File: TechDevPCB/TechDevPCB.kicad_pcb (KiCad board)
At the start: 2 copper layers, 80.8 x 104.3 mm, 51 parts, among them J1 Screw_Terminal_01x02, J10 Conn_01x05_Pin, J11 Conn_01x01_Socket, J12 Screw_Terminal_01x04, J13 Conn_01x01_Socket, J14 Conn_01x01_Socket, J15 Conn_01x01_Socket, J16 Conn_01x01_Socket, J17 Conn_01x01_Socket, J18 Conn_01x01_Socket, J19 Conn_01x01_Socket, J2 Screw_Terminal_01x02, J20 Conn_01x01_Socket, J21 Conn_01x01_Socket, J22 Conn_01x01_Socket, J23 Conn_01x01_Socket, J24 Conn_01x01_Socket, J25 Conn_01x01_Socket, J26 Conn_01x01_Socket, J27 Conn_01x01_Socket, J28 Conn_01x01_Socket, J29 Conn_01x01_Socket, J3 Conn_01x02_Pin, J30 Conn_01x01_Socket, J31 Conn_01x01_Socket, J4 Screw_Terminal_01x04, J5 Conn_01x02_Pin, J6 Conn_01x05_Pin, J7 Conn_01x04_Pin, J8 Conn_01x05_Pin, J9 Conn_01x05_Pin, U1 DRV8825_STEPPER_MOTOR_DRIVER_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, U2 DRV8825_STEPPER_MOTOR_DRIVER_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, U3 XL6009 Boost Converter

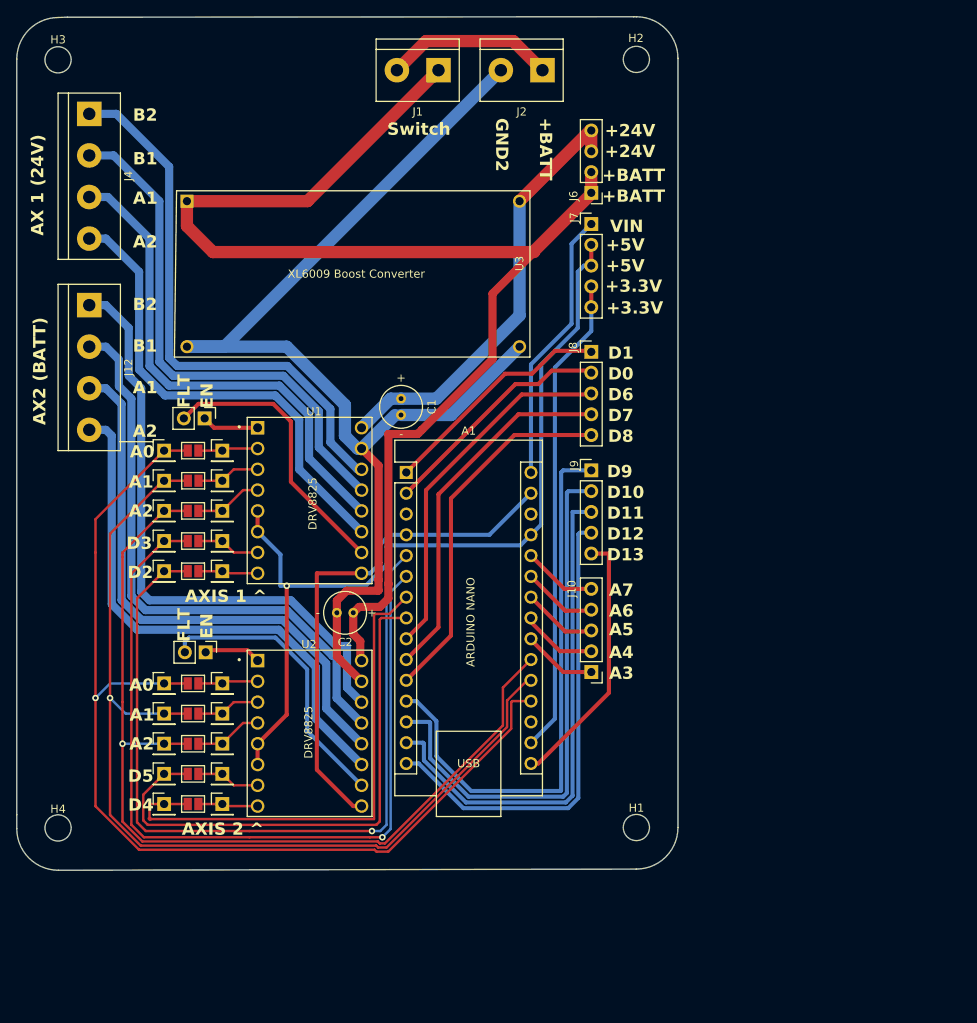
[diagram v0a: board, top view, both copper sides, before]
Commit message: PCB Updates
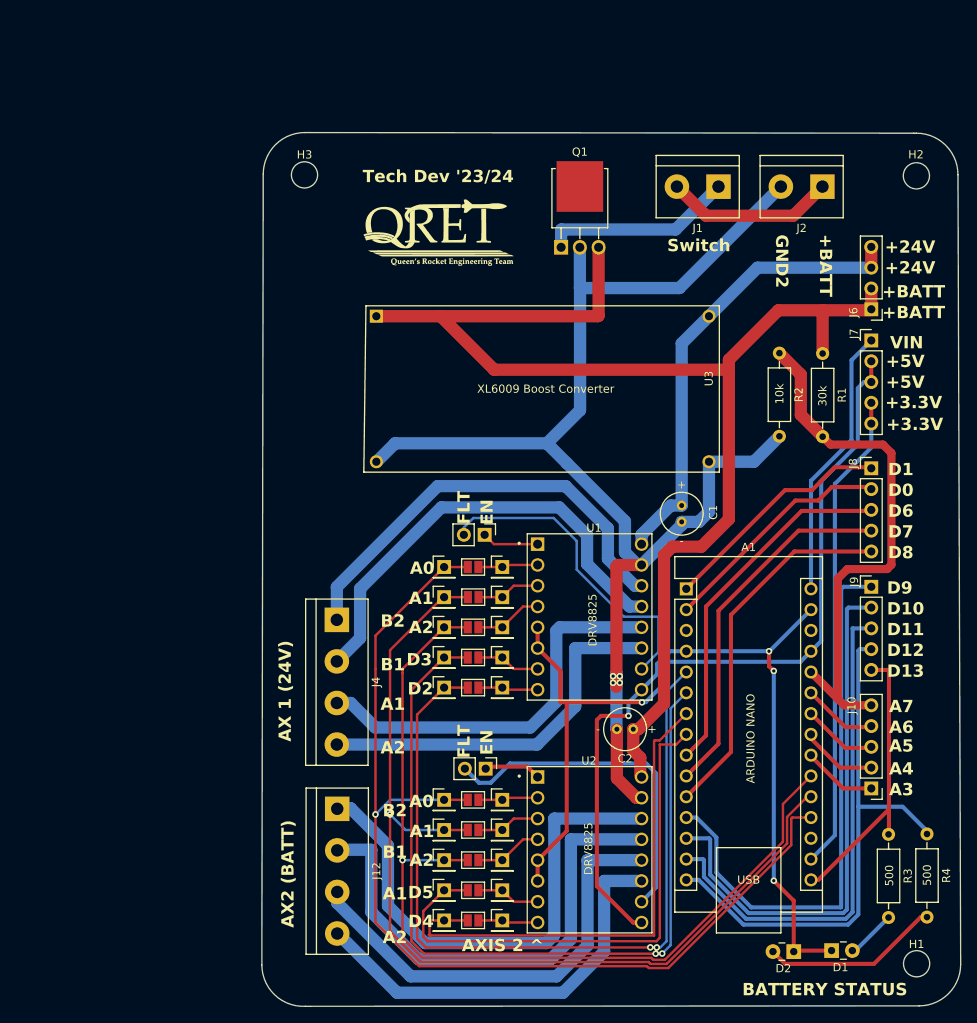
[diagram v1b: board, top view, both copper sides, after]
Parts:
- removed H4: MountingHole, MountingHole:MountingHole_3.2mm_M3_DIN965
- added D1: LED, LED_THT:LED_Rectangular_W3.0mm_H2.0mm, F.Cu at (174.0, 138.0)
- added D2: LED, LED_THT:LED_Rectangular_W3.0mm_H2.0mm, F.Cu at (169.4, 138.2)
- added G***: LOGO, Footprints:QRET, F.Cu at (125.4, 50.8)
- added Q1: PMOS, Package_TO_SOT_THT:TO-251-3-1EP_Horizontal_TabDown, F.Cu at (141.0, 52.1)
- added R1: 30k, Resistor_THT:R_Axial_DIN0207_L6.3mm_D2.5mm_P10.16mm_Horizontal, F.Cu at (172.9, 65.1)
- added R2: 10k, Resistor_THT:R_Axial_DIN0207_L6.3mm_D2.5mm_P10.16mm_Horizontal, F.Cu at (167.6, 65.0)
- added R3: 500, Resistor_THT:R_Axial_DIN0207_L6.3mm_D2.5mm_P10.16mm_Horizontal, F.Cu at (181.0, 123.9)
- added R4: 500, Resistor_THT:R_Axial_DIN0207_L6.3mm_D2.5mm_P10.16mm_Horizontal, F.Cu at (185.7, 123.8)
- moved J4 68.8 mm to (113.6, 97.6)
- moved J12 68.6 mm to (113.6, 120.7)
- moved H1 38.1 mm to (184.4, 139.7)
- moved C2 37.1 mm to (149.8, 111.0)
- moved J9 37.1 mm to (178.9, 93.6)
- moved J10 37.1 mm to (178.9, 118.2)
- moved J29 37.1 mm to (133.8, 134.4)
- moved J6 37.1 mm to (178.9, 63.5)
- moved J7 37.1 mm to (178.9, 59.7)
- moved J8 37.1 mm to (178.9, 79.1)
- moved JP9 37.1 mm to (130.2, 134.4)
- moved J1 37.1 mm to (160.2, 44.7)
- moved J13 37.1 mm to (133.8, 91.2)
- moved J15 37.1 mm to (133.8, 94.9)
- moved J17 37.1 mm to (133.8, 98.6)
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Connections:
- J1 pad 1: +BATT -> Net-(J1-Pin_1)
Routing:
- net A7: track 9.05 -> 66.4 mm
- net GND: track 62.9 -> 103.8 mm, vias 0 -> 4
- net Net-(J1-Pin_1): track 0.00 -> 23.6 mm
- net Net-(D2-A): track 0.00 -> 21.8 mm
- net GND2: track 140.4 -> 159.7 mm, vias 0 -> 4
- net AX2_A2: track 66.0 -> 50.9 mm
- net AX2_A1: track 68.5 -> 54.2 mm
- net AX1_B2: track 67.3 -> 53.6 mm
- net AX1_A1: track 61.4 -> 48.6 mm
- net AX1_A2: track 58.7 -> 46.3 mm
- net AX2_B2: track 74.3 -> 63.0 mm
- net AX2_B1: track 71.4 -> 60.4 mm
- net D12: track 57.7 -> 67.7 mm
- net AX1_B1: track 64.3 -> 55.7 mm
- net AX2_FLT: track 35.0 -> 42.0 mm
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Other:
- board size 80.8 x 104.3 mm -> 85.4 x 106.8 mm
- board text added: "10k"
- board text added: "500"
- board text added: "BATTERY STATUS"
- board text added: "Tech Dev '23/24"
- board text removed: "AXIS 1 ^"
